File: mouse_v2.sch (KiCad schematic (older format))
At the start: 98 parts, among them J1 HC05 Header, J2 Serial Debug Header, J3 HC05_Key Jump, J4 Conn_ARM_JTAG_SWD_10, J5 SWD Header, M1 M1_Conn, M2 M2_Conn, M3 M1_Conn_Alt, M4 M2_Conn_Alt, Q0 Q_Photo_NPN, Q1 Q_Photo_NPN, Q2 Q_Photo_NPN, Q3 Q_Photo_NPN, Q4 Q_NMOS_SGD, Q5 Q_NMOS_SGD, Q6 Q_NMOS_SGD, Q7 Q_NMOS_SGD, Q8 Q_NMOS_SGD, SW1 SW, U1 YAAJ_BluePill_SWD_Breakout, U2 L293D, U3 LM1085-5.0, U4 APE8865Y5-33-HF-3

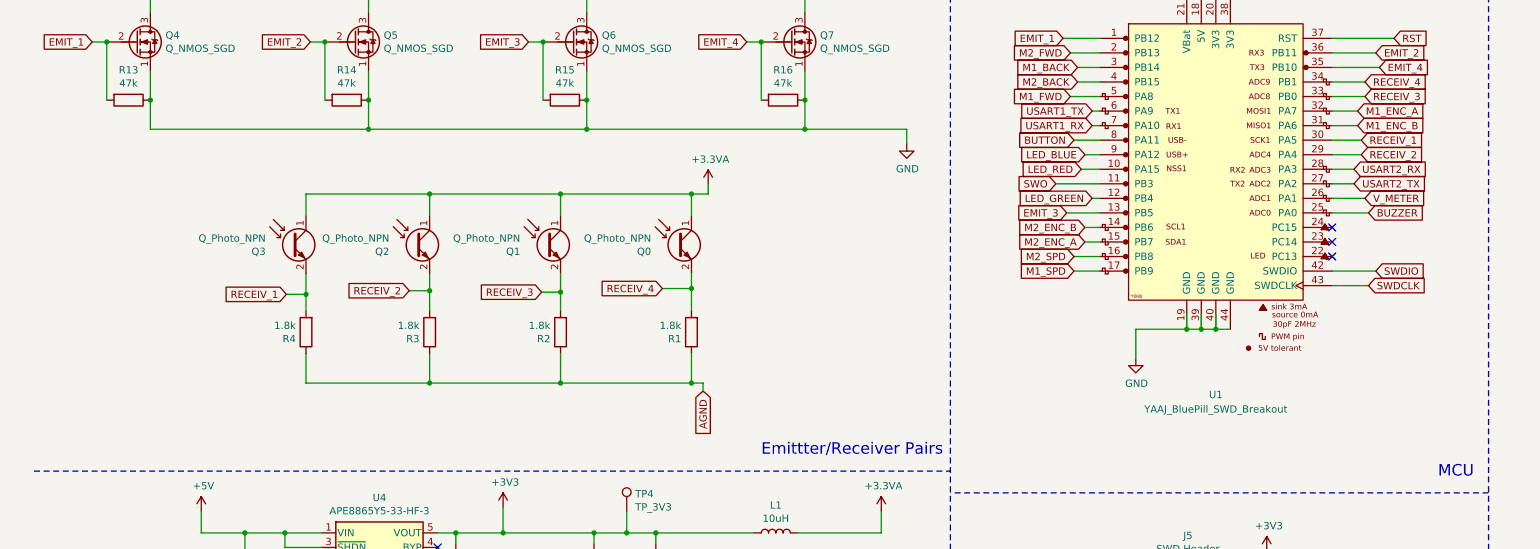
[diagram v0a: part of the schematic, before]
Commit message: tracing
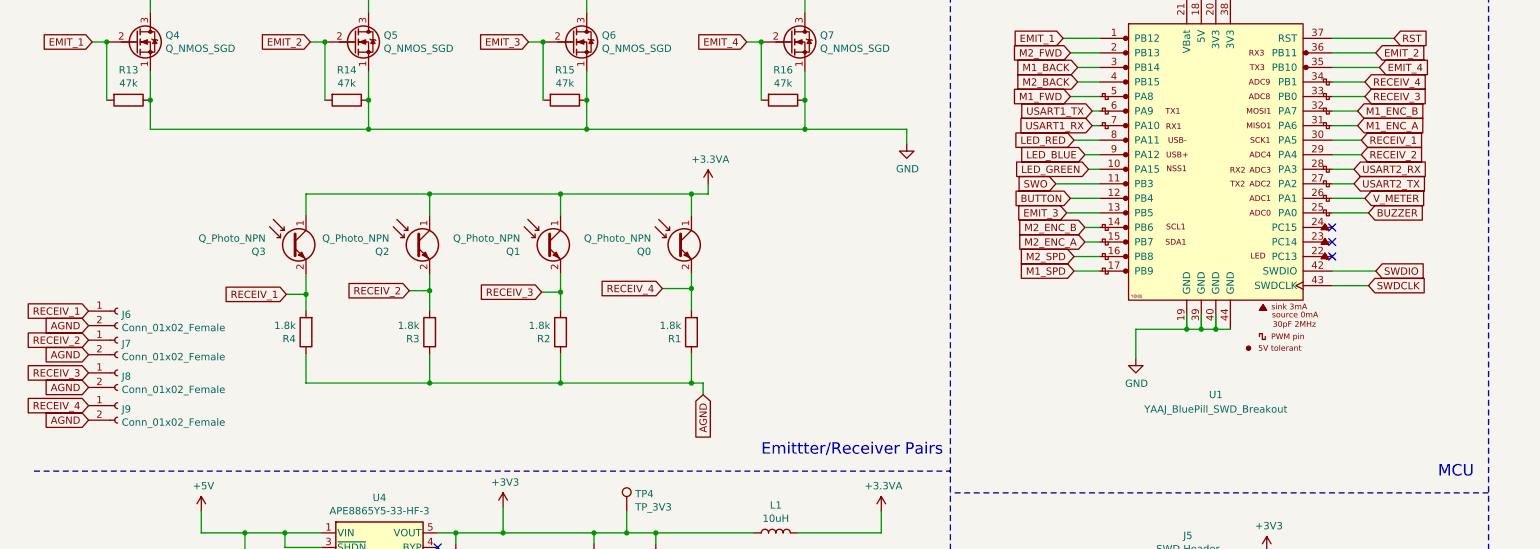
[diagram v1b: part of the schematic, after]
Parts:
- added J6, J7, J8, J9: Conn_01x02_Female, Connector_PinSocket_2.00mm:PinSocket_1x02_P2.00mm_Vertical, symbol Connector:Conn_01x02_Female
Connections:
- net AGND: now also J6.2 (Pin_2), J7.2 (Pin_2), J8.2 (Pin_2), J9.2 (Pin_2)
- net BUTTON: now also U1.12 (PB4); no longer U1.8 (PA11)
- net LED_GREEN: now also U1.10 (PA15); no longer U1.12 (PB4)
- net LED_RED: now also U1.8 (PA11); no longer U1.10 (PA15)
- net M1_ENC_A: now also U1.31 (PA6); no longer U1.32 (PA7)
- net M1_ENC_B: now also U1.32 (PA7); no longer U1.31 (PA6)
- net RECEIV_1: now also J6.1 (Pin_1)
- net RECEIV_2: now also J7.1 (Pin_1)
- net RECEIV_3: now also J8.1 (Pin_1)
- net RECEIV_4: now also J9.1 (Pin_1)
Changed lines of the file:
@@
 Text GLabel 7775 2475 0    50   Input ~ 0
 USART1_TX
-Text GLabel 7650 2675 0    50   Input ~ 0
+Text GLabel 7625 3075 0    50   Input ~ 0
 BUTTON
 Text GLabel 7675 2275 0    50   Input ~ 0
@@
 Text GLabel 7600 3175 0    50   Input ~ 0
 EMIT_3
-Text GLabel 7775 3075 0    50   Input ~ 0
+Text GLabel 7750 2875 0    50   Input ~ 0
 LED_GREEN
-Text GLabel 7700 2875 0    50   Input ~ 0
+Text GLabel 7650 2675 0    50   Input ~ 0
 LED_RED
+Text GLabel 9600 2475 2    50   Input ~ 0
+M1_ENC_B
 Text GLabel 9600 2575 2    50   Input ~ 0
-M1_ENC_B
-Text GLabel 9600 2475 2    50   Input ~ 0
 M1_ENC_A
 Text GLabel 7650 3575 0    50   Input ~ 0
@@
 	7825 2575 7775 2575
 Wire Wire Line
-	7825 3075 7775 3075
-Wire Wire Line
 	7825 3275 7725 3275
 Wire Wire Line
@@
 Wire Wire Line
 	5020 4345 5100 4345
-Wire Wire Line
-	5100 4345 5100 4405
 Connection ~ 5020 4345
 $Comp
@@
 Wire Wire Line
 	6100 7575 5975 7575
-Text GLabel 5100 4400 3    50   Input ~ 0
+Text GLabel 5100 4425 3    50   Input ~ 0
 AGND
 Wire Wire Line
@@
 	8975 5575 8975 5500
 Wire Wire Line
-	7825 2875 7700 2875
-Wire Wire Line
 	7600 3175 7825 3175
 Wire Wire Line
@@
 	7825 2775 7725 2775
 Wire Wire Line
+	7575 1975 7825 1975
+Wire Wire Line
+	7825 2075 7625 2075
+Wire Wire Line
+	7675 2175 7825 2175
+Wire Wire Line
+	7825 2275 7675 2275
+Wire Wire Line
+	7625 2375 7825 2375
+$Comp
+L Connector:Conn_01x02_Female J6
+U 1 1 635B9403
+P 1075 3850
+F 0 "J6" H 1103 3826 50  0000 L CNN
+F 1 "Conn_01x02_Female" H 1103 3735 50  0000 L CNN
+F 2 "Connector_PinSocket_2.00mm:PinSocket_1x02_P2.00mm_Vertical" H 1075 3850 50  0001 C CNN
+F 3 "~" H 1075 3850 50  0001 C CNN
+	1    1075 3850
+	1    0    0    -1
+$EndComp
+$Comp
+L Connector:Conn_01x02_Female J7
+U 1 1 635BB2ED
+P 1075 4050
+F 0 "J7" H 1103 4026 50  0000 L CNN
+F 1 "Conn_01x02_Female" H 1103 3935 50  0000 L CNN
+F 2 "Connector_PinSocket_2.00mm:PinSocket_1x02_P2.00mm_Vertical" H 1075 4050 50  0001 C CNN
+F 3 "~" H 1075 4050 50  0001 C CNN
+	1    1075 4050
+	1    0    0    -1
+$EndComp
+$Comp
+L Connector:Conn_01x02_Female J8
+U 1 1 635BB64C
+P 1075 4275
+F 0 "J8" H 1103 4251 50  0000 L CNN
+F 1 "Conn_01x02_Female" H 1103 4160 50  0000 L CNN
+F 2 "Connector_PinSocket_2.00mm:PinSocket_1x02_P2.00mm_Vertical" H 1075 4275 50  0001 C CNN
+F 3 "~" H 1075 4275 50  0001 C CNN
+	1    1075 4275
+	1    0    0    -1
+$EndComp
+$Comp
+L Connector:Conn_01x02_Female J9
+U 1 1 635BBA41
+P 1075 4500
+F 0 "J9" H 1103 4476 50  0000 L CNN
+F 1 "Conn_01x02_Female" H 1103 4385 50  0000 L CNN
+F 2 "Connector_PinSocket_2.00mm:PinSocket_1x02_P2.00mm_Vertical" H 1075 4500 50  0001 C CNN
+F 3 "~" H 1075 4500 50  0001 C CNN
+	1    1075 4500
+	1    0    0    -1
+$EndComp
+Text GLabel 875  3850 0    50   Input ~ 0
+RECEIV_1
+Text GLabel 875  4050 0    50   Input ~ 0
+RECEIV_2
+Text GLabel 875  4275 0    50   Input ~ 0
+RECEIV_3
+Text GLabel 875  4500 0    50   Input ~ 0
+RECEIV_4
+Text GLabel 875  3950 0    50   Input ~ 0
+AGND
+Text GLabel 875  4150 0    50   Input ~ 0
+AGND
+Text GLabel 875  4375 0    50   Input ~ 0
+AGND
+Text GLabel 875  4600 0    50   Input ~ 0
+AGND
+Wire Wire Line
+	5100 4345 5100 4425
+Wire Wire Line
+	7625 3075 7825 3075
+Wire Wire Line
+	7750 2875 7825 2875
+Wire Wire Line
 	7825 2675 7650 2675
-Wire Wire Line
-	7575 1975 7825 1975
-Wire Wire Line
-	7825 2075 7625 2075
-Wire Wire Line
-	7675 2175 7825 2175
-Wire Wire Line
-	7825 2275 7675 2275
-Wire Wire Line
-	7625 2375 7825 2375
 $EndSCHEMATC
